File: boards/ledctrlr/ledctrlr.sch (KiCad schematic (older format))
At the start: 56 parts, among them IC1 ATMEGA168-P, IC2 SN75176B, J1 RJ45, J2 RJ45, SW1 SW_PUSH, U1 LM7805, X1 CRYSTAL

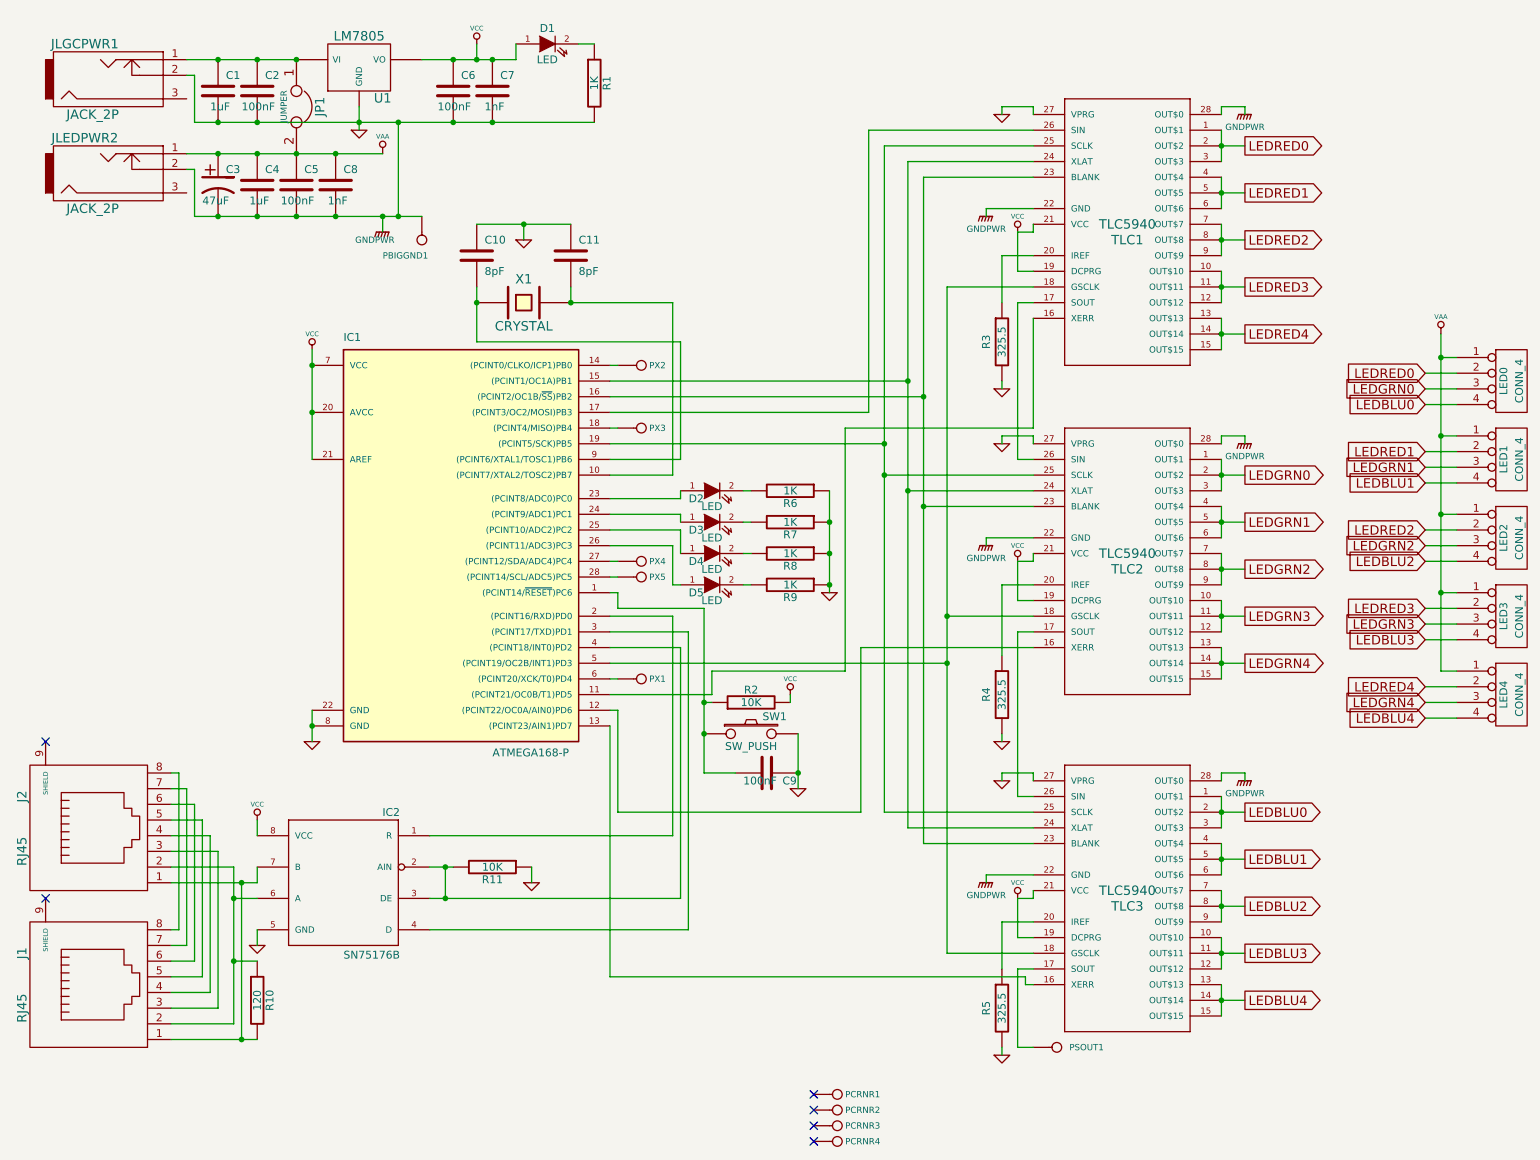
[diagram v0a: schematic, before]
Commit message: placement of v2.0 boards almost done
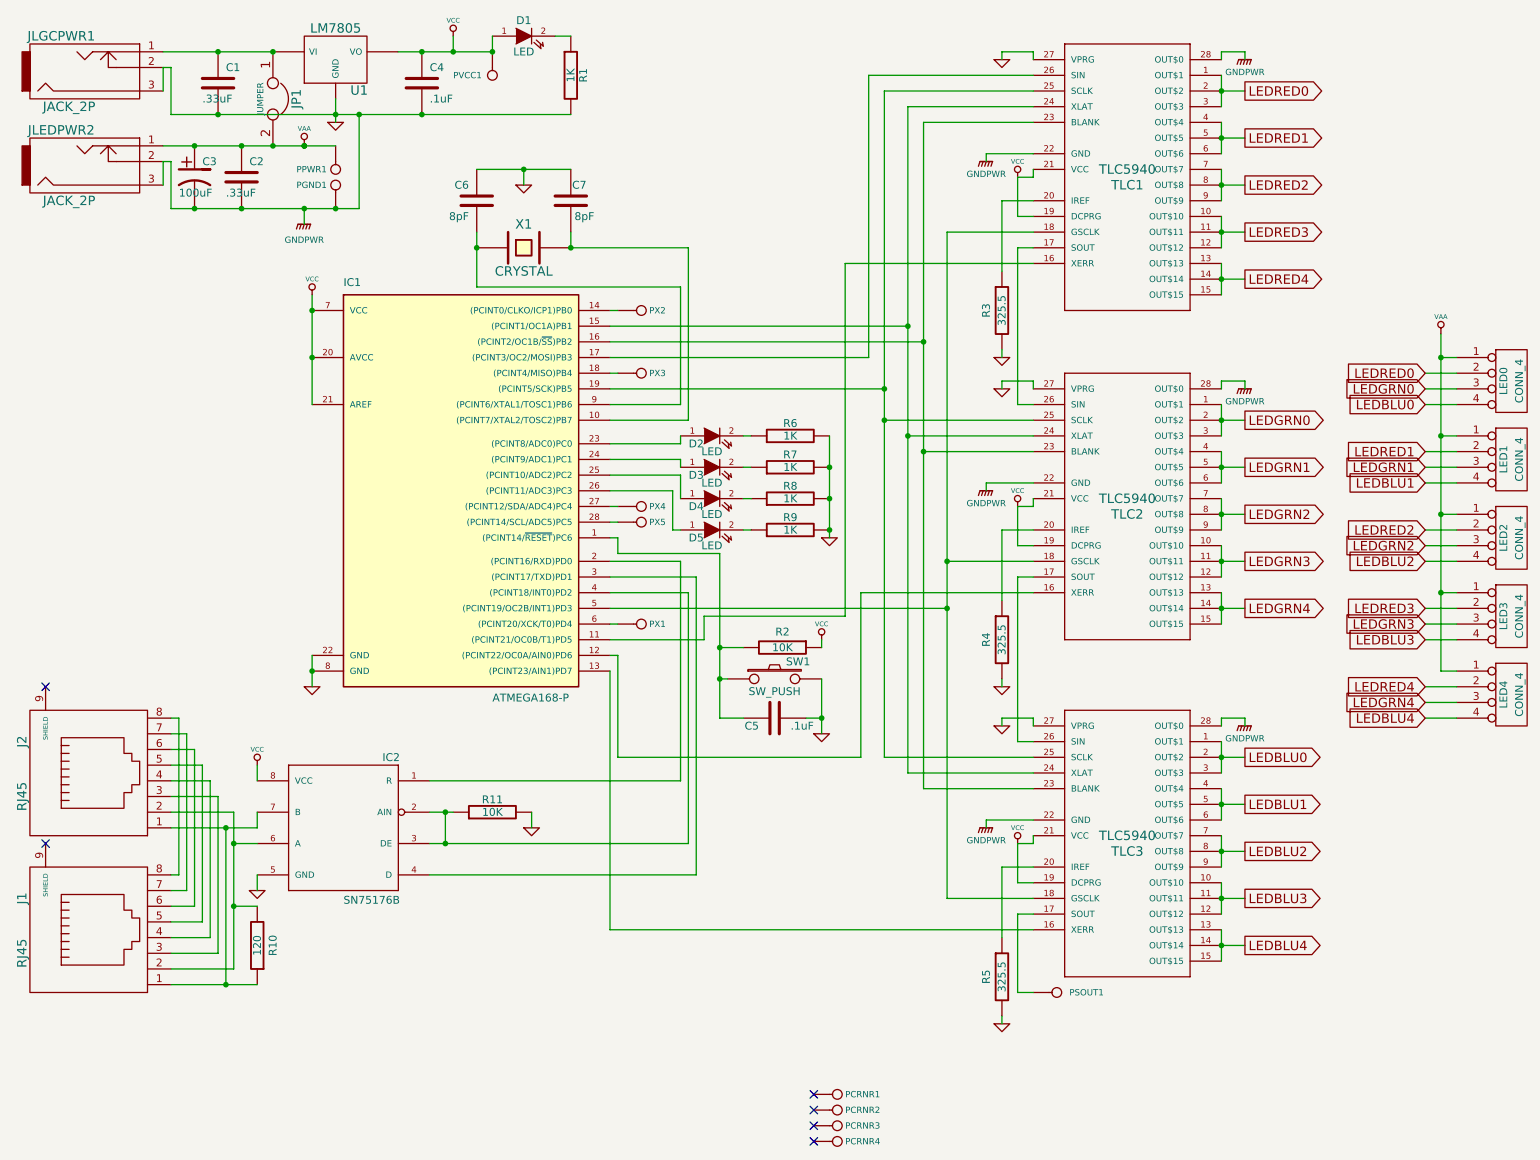
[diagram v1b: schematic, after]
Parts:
- removed C1: 1uF, C1, symbol C
- removed C11: 8pF, SM0805, symbol C
- removed C6: 100nF, C1, symbol C
- removed C8: 1nF, C1, symbol C
- removed C9: 100nF, SM0805, symbol C
- added C2: .33uF, SM0805, symbol C
- added PPWR1, PVCC1: CONN_1, PAD, symbol CONN_1
- C1: renamed from C2; value 100nF -> .33uF; footprint C1 -> SM0805; DigikeyPart 478-4862-ND -> 445-1356-1-ND; Part SR215C103KAR -> C2012X7R1C334K/1.25
- C3: value 47uF -> 100uF; DigikeyPart P5137-ND -> 399-6103-ND; Part ECA-1CM470 -> ESK107M025AE3AA
- C4: value 1uF -> .1uF; footprint C1 -> SM0805; DigikeyPart 478-5812-ND -> 311-1361-1-ND; Part TAP105M035SCS -> CC0805ZRY5V9BB104
- C5: value 100nF -> .1uF; footprint C1 -> SM0805; DigikeyPart 478-1831-ND -> 311-1361-1-ND; Part TAP104K035SCS -> CC0805ZRY5V9BB104
- C6: renamed from C10; Part CC0805DRNP09BN8R0 -> CC0805DRNPO9BN8R0
- C7: value 1nF -> 8pF; footprint C1 -> SM0805; DigikeyPart 478-4862-ND -> 311-1097-1-ND; Part SR215C103KAR -> CC0805DRNPO9BN8R0
- D1, D2, D3, D4, D5: footprint LED-1206 -> LED-1206-3D
- IC2: footprint DIP-8__300 -> SOIC8
- LED0, LED1, LED2, LED3, LED4: footprint (none) -> OSTTA040161
- PGND1: renamed from PBIGGND1; footprint 1pin -> PAD
- PSOUT1, PX1, PX2, PX3, PX4, PX5: footprint SIL-1 -> PAD
- R11: footprint (none) -> SM0805
- TLC1, TLC2, TLC3: footprint DIP-28__300 -> tssop-28-thermal
- U1: footprint LM78XXV -> LM78XXV-3D
- X1: footprint Crystal_FOX-FE-SMD-RevA_09Aug201 -> Crystal_FOX-FE_SMD_RevA_09Aug2010
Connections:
- net GND: now also C6.2, JLEDPWR2.3, JLGCPWR1.3, R11.2, R6.2, R7.2, R8.2, R9.2, C2.2; no longer C6.1, R11.1, R6.1, R7.1, R8.1, R9.1
- net VAA: now also C2.1, PPWR1.1; no longer C4.1, C5.1
- net VCC: now also C4.1, R2.1, PVCC1.1; no longer C7.1, R2.2
- net at IC1.4 ((PCINT18/INT0)PD2), IC2.2 (AIN), IC2.3 (DE): now also R11.1; no longer R11.2
- net at IC2.6 (A), J1.2, J2.2: now also R10.2; no longer R10.1
- net at IC2.7 (B), J1.1, J2.1: now also R10.1; no longer R10.2
- net at IC1.9 ((PCINT6/XTAL1/TOSC1)PB6), X1.1: now also C6.1; no longer C6.2
- net at IC1.10 ((PCINT7/XTAL2/TOSC2)PB7), X1.2: now also C7.1
- net at IC1.1 ((PCINT14/~RESET~)PC6), SW1.1: now also C5.1, R2.2; no longer R2.1
- net at D2.2 (K): now also R6.1; no longer R6.2
- net at D3.2 (K): now also R7.1; no longer R7.2
- net at D4.2 (K): now also R8.1; no longer R8.2
- net at D5.2 (K): now also R9.1; no longer R9.2
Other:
- moved on the sheet: C1, C3, C6, D1, D2, D3, D4, D5, IC1, IC2, J1, J2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
